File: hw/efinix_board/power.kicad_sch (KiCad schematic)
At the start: 55 parts, among them U1 T20F256, U2 TPS62826, U3 TPS62826

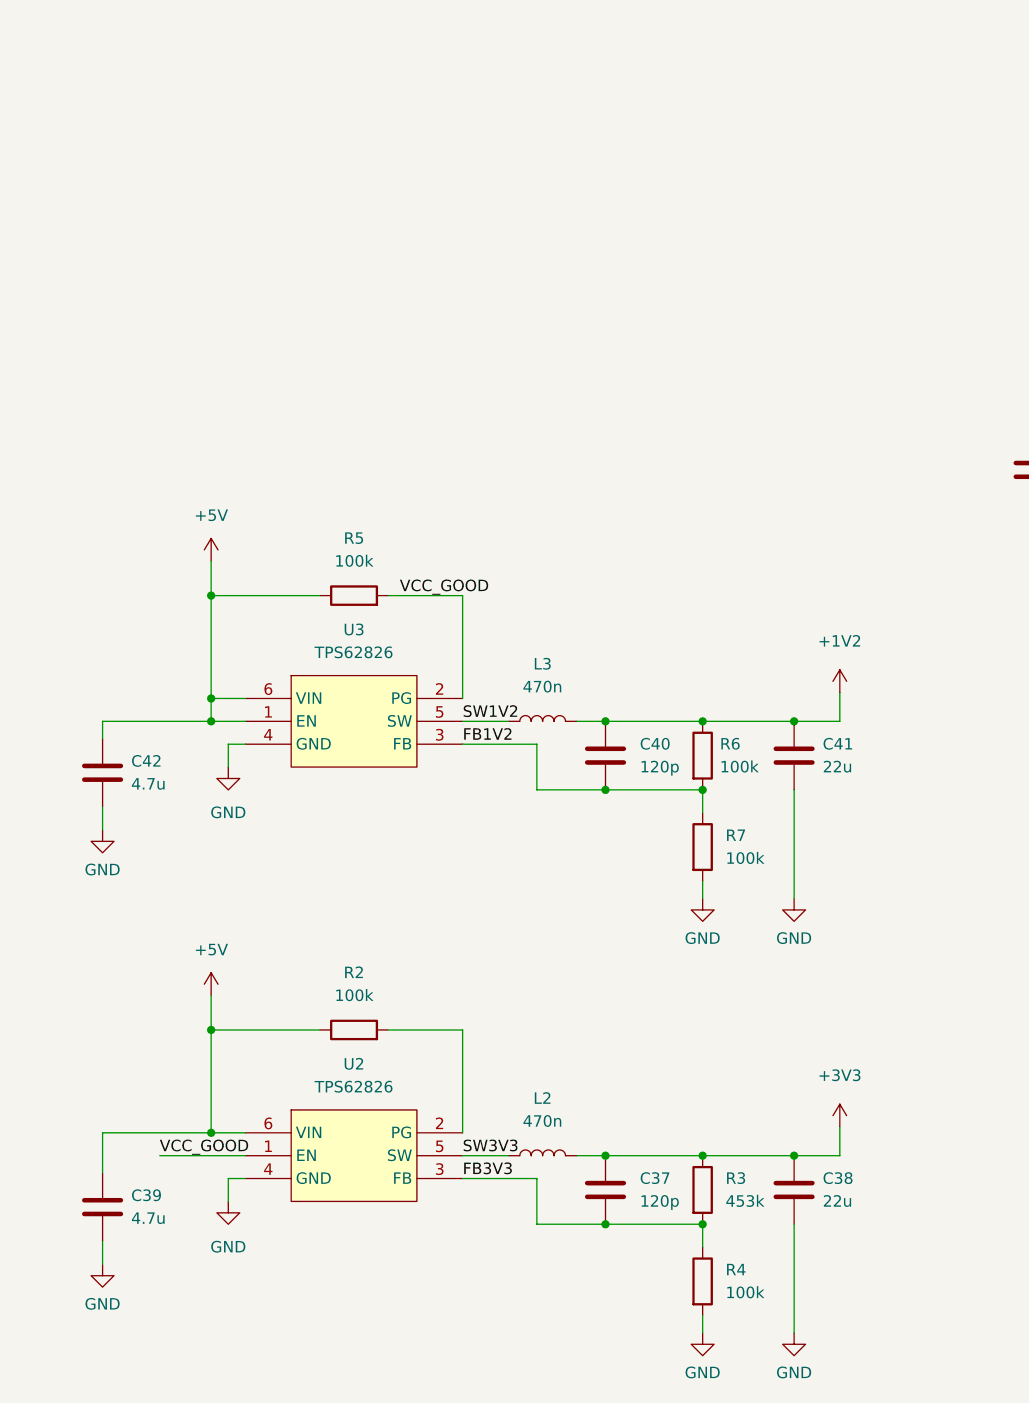
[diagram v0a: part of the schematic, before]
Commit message: Start working on sdram
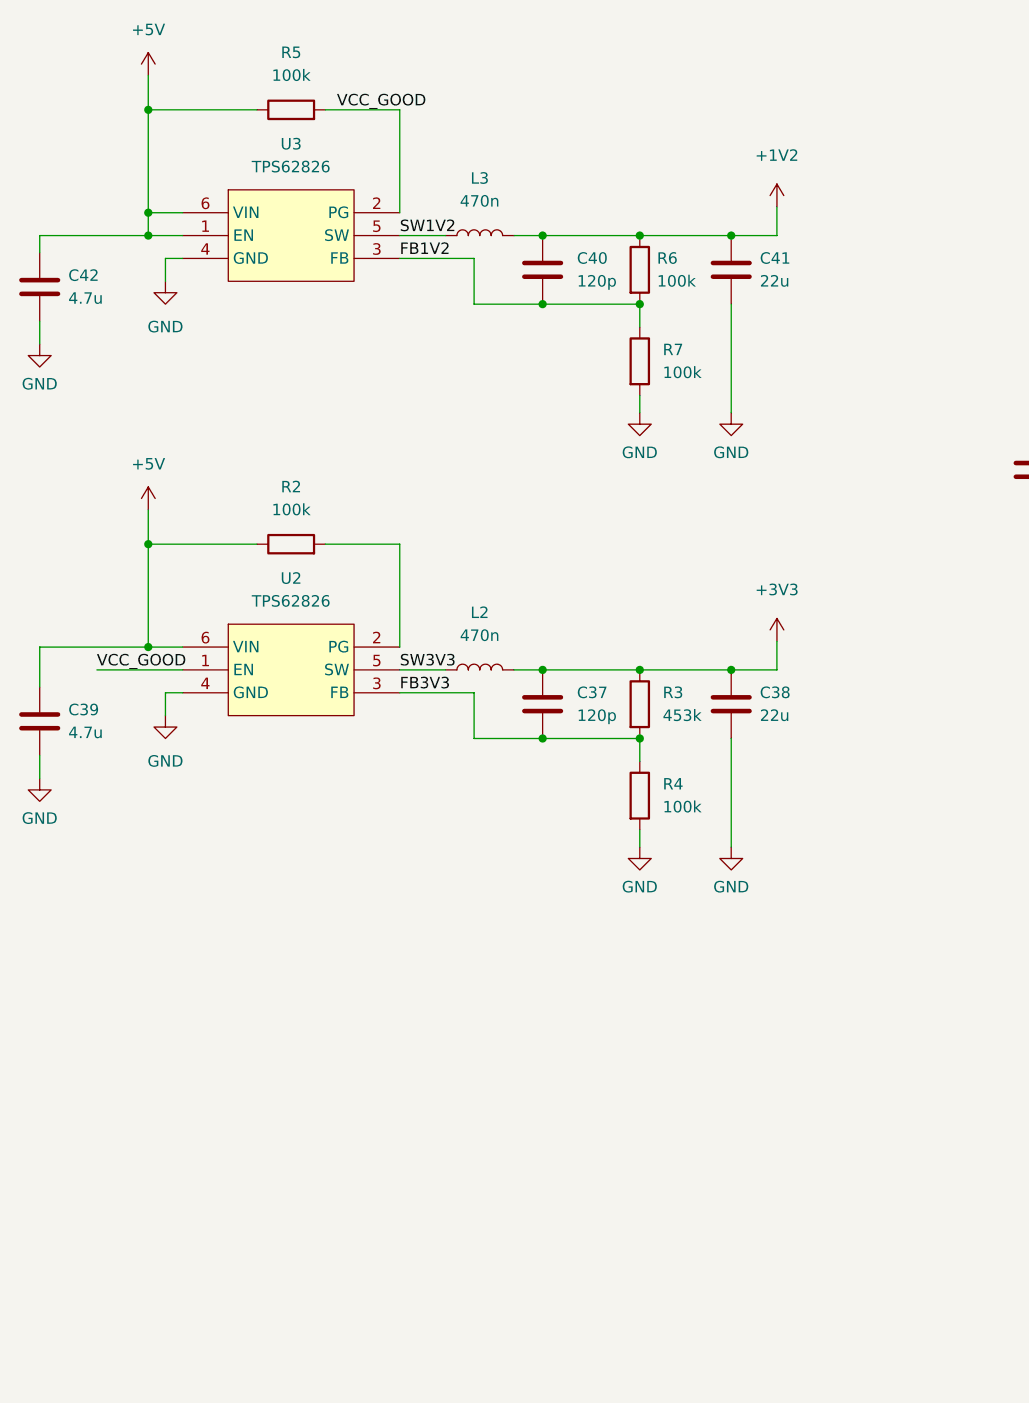
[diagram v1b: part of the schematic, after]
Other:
- moved on the sheet: C37, C38, C39, C40, C41, C42, L2, L3, R2, R3, R4, R5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
